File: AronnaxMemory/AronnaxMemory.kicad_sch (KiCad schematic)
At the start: 35 parts, among them J1 Barrel_Jack_Switch, J12 Conn_02x08_Odd_Even, J13 Conn_02x18_Odd_Even, J2 Conn_02x40_Odd_Even, J3 Conn_02x18_Odd_Even, J8 Conn_02x10_Odd_Even, J9 VP A1-A4, U10 ATF22V10, U4 ATF22V10, U5 74LS348, U9 ATF22V10

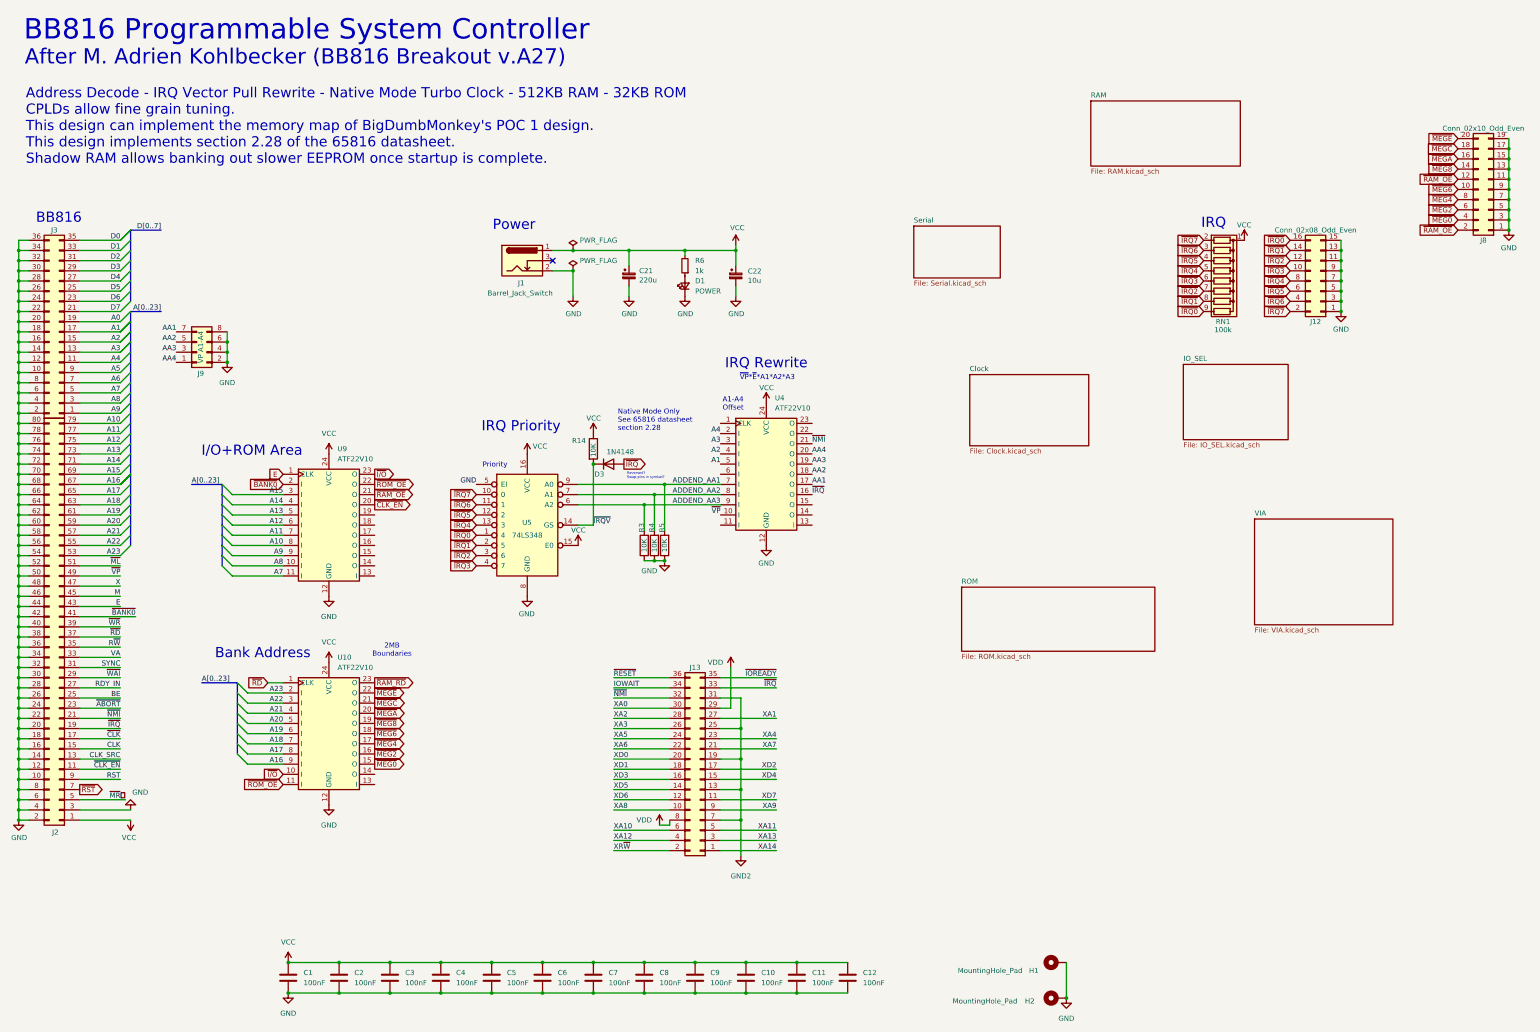
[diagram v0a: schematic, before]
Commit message: All of it p2
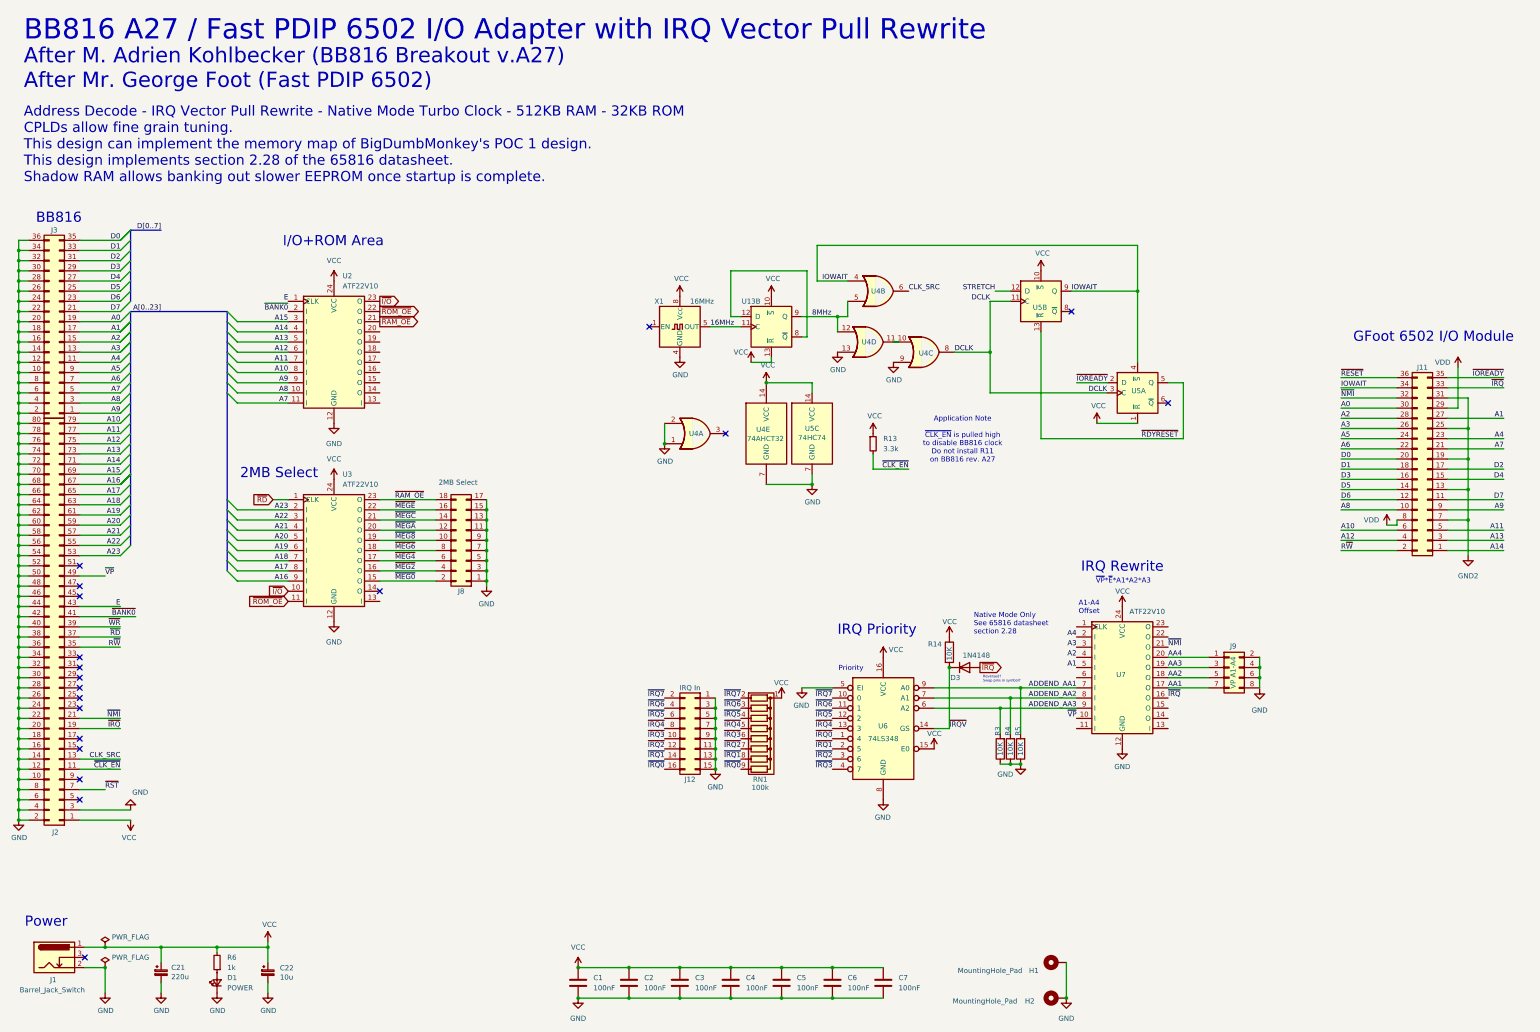
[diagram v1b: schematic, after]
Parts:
- removed C10, C11, C12, C8, C9: 100nF, Capacitor_THT:C_Disc_D3.4mm_W2.1mm_P2.50mm, symbol Device:C
- removed J13: Conn_02x18_Odd_Even, PCB_Edge_Connectors:PCB_Edge_36pin, symbol Connector_Generic:Conn_02x18_Odd_Even
- added J11: Conn_02x18_Odd_Even, PCB_Edge_Connectors:PCB_Edge_36pin, symbol Connector_Generic:Conn_02x18_Odd_Even
- added R13: 3.3k, Resistor_THT:R_Axial_DIN0207_L6.3mm_D2.5mm_P7.62mm_Horizontal, symbol Device:R_Small
- added U13, U5: 74HC74, Package_DIP:DIP-14_W7.62mm, symbol 74xx:74LS74
- added U4: 74AHCT32, Package_DIP:DIP-14_W7.62mm_Socket, symbol AronnaxLibrary:74AHCT32
- added X1: 16MHz, Oscillator:Oscillator_DIP-8, symbol Oscillator:CXO_DIP8
- J12: value Conn_02x08_Odd_Even -> IRQ In
- J8: value Conn_02x10_Odd_Even -> 2MB Select; footprint Connector_PinHeader_2.54mm:PinHeader_2x10_P2.54mm_Vertical -> Connector_PinHeader_2.54mm:PinHeader_2x09_P2.54mm_Vertical; symbol Connector_Generic:Conn_02x10_Odd_Even -> Connector_Generic:Conn_02x09_Odd_Even
- renumbered U9 to U2, U10 to U3, U5 to U6, U4 to U7
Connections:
- net ~{RAM_RD} is gone; now on net ~{RAM_OE}: U3.23 (O)
- net A0: now also J11.30 (Pin_30)
- net A1: now also J11.27 (Pin_27)
- net A10: now also J11.6 (Pin_6)
- net A11: now also J11.5 (Pin_5)
- net A12: now also J11.4 (Pin_4)
- net A13: now also J11.3 (Pin_3)
- net A14: now also J11.1 (Pin_1)
- net A2: now also J11.28 (Pin_28)
- net A3: now also J11.26 (Pin_26)
- net A4: now also J11.23 (Pin_23)
- net A5: now also J11.24 (Pin_24)
- net A6: now also J11.22 (Pin_22)
- net A7: now also J11.21 (Pin_21)
- net A8: now also J11.10 (Pin_10)
- net A9: now also J11.9 (Pin_9)
- net CLK_SRC: now also U4.6
- net D0: now also J11.20 (Pin_20)
- net D1: now also J11.18 (Pin_18)
- net D2: now also J11.17 (Pin_17)
- net D3: now also J11.16 (Pin_16)
- net D4: now also J11.15 (Pin_15)
- net D5: now also J11.14 (Pin_14)
- net D6: now also J11.12 (Pin_12)
- net D7: now also J11.11 (Pin_11)
- net GND: now also U4.1, U4.13, U4.2, U4.7 (GND), U4.9, U5.7 (GND), X1.4 (GND); no longer J8.19 (Pin_19), J9.2 (Pin_2), J9.4 (Pin_4), J9.6 (Pin_6), J9.8 (Pin_8)
- net GND2: now also J11.13 (Pin_13), J11.19 (Pin_19), J11.25 (Pin_25), J11.31 (Pin_31), J11.7 (Pin_7)
- net IOWAIT: now also J11.34 (Pin_34), U4.4, U5.4 (~{S}), U5.9 (Q)
- net R~{W}: now also J11.2 (Pin_2)
- net VCC: now also R13.1, U13.10 (~{S}), U13.13 (~{R}), U4.14 (VCC), U5.1 (~{R}), U5.10 (~{S}), U5.14 (VCC), X1.8 (Vcc)
- net VDD: now also J11.29 (Pin_29), J11.8 (Pin_8)
- net ~{CLK_EN}: now also R13.2; no longer U2.20 (O)
- net ~{IOREADY}: now also J11.35 (Pin_35), U5.2 (D)
- net ~{IRQ}: now also J11.33 (Pin_33)
- net ~{MEG0}: now also J8.2 (Pin_2); no longer J8.4 (Pin_4)
- net ~{MEG2}: now also J8.4 (Pin_4); no longer J8.6 (Pin_6)
- net ~{MEG4}: now also J8.6 (Pin_6); no longer J8.8 (Pin_8)
- net ~{MEG6}: now also J8.8 (Pin_8); no longer J8.10 (Pin_10)
- net ~{MEG8}: now also J8.10 (Pin_10); no longer J8.14 (Pin_14)
- net ~{MEGA}: now also J8.12 (Pin_12); no longer J8.16 (Pin_16)
- net ~{MEGC}: now also J8.14 (Pin_14); no longer J8.18 (Pin_18)
- net ~{MEGE}: now also J8.16 (Pin_16); no longer J8.20 (Pin_20)
- net ~{NMI}: now also J11.32 (Pin_32)
- net ~{RAM_OE}: now also J8.18 (Pin_18); no longer J8.12 (Pin_12), J8.2 (Pin_2)
- net ~{RESET}: now also J11.36 (Pin_36)
- net BE: no longer names the net of J2.25 (Pin_25)
- net CLK: no longer names the net of J2.15 (Pin_15)
- net M: no longer names the net of J2.45 (Pin_45)
- net RDY_IN: no longer names the net of J2.27 (Pin_27)
- net RST: no longer names the net of J2.9 (Pin_9)
- net SYNC: no longer names the net of J2.31 (Pin_31)
- net VA: no longer names the net of J2.33 (Pin_33)
- net X: no longer names the net of J2.47 (Pin_47)
- net ~{ABORT}: no longer names the net of J2.23 (Pin_23)
- net ~{CLK}: no longer names the net of J2.17 (Pin_17)
- net ~{ML}: no longer names the net of J2.51 (Pin_51)
- net ~{MR}⎒: no longer names the net of J2.5 (Pin_5)
- net ~{WAI}: no longer names the net of J2.29 (Pin_29)
- new net: J9.2 (Pin_2), J9.4 (Pin_4), J9.6 (Pin_6), J9.8 (Pin_8)
- new net: U4.10, U4.11
- new net: U13.12 (D), U13.8 (~{Q})
- new net 16MHz: U13.11 (C), X1.5 (OUT)
- new net 8MHz: U13.9 (Q), U4.12, U4.5
- new net DCLK: U4.8, U5.11 (C), U5.3 (C)
- new net STRETCH: U5.12 (D)
- new net ~{RDYRESET}: U5.13 (~{R}), U5.5 (Q)
- no-connect marks 1 -> 19
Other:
- removed sheet Clock
- removed sheet IO_SEL
- removed sheet RAM
- removed sheet ROM
- removed sheet Serial
- removed sheet VIA
- note added: "2MB Select"
- note added: "After M. Adrien Kohlbecker (BB816 Breakout v.A27) After Mr. George Foot (Fast PDIP 6502)"
- note added: "Application Note ~{CLK_EN} is pulled high to disable BB816 clock Do not install R11 on BB816 rev. A27"
- note added: "BB816 A27 / Fast PDIP 6502 I/O Adapter with IRQ Vector Pull Rewrite"
- note added: "GFoot 6502 I/O Module"
- note removed: "2MB Boundaries"
- note removed: "After M. Adrien Kohlbecker (BB816 Breakout v.A27)"
- note removed: "BB816 Programmable System Controller"
- note removed: "Bank Address"
- note removed: "IRQ"
- moved on the sheet: C1, C2, C21, C22, C3, C4, C5, C6, C7, D1, D3, J1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
